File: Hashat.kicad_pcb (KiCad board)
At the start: 4 copper layers, 65 x 56.5 mm, 109 parts, among them IC1 BM1397_mode1, J1 Raspberry_Pi_2_3, J2 Conn_01x04, J3 Conn_01x05, Q1 CSD17311Q5, Q2 CSD17311Q5, U10 DS4432U+, U2 LN1134A182MR-G, U3 SN74LVC1T45DBVR, U4 SGM2036-ADJYN5G/TR, U5 SN74LVC1T45DBVR, U7 EMC2101-R, U8 SN74LVC1T45DBVR, U9 TPS40305, X1 OT322525MJBA4SL

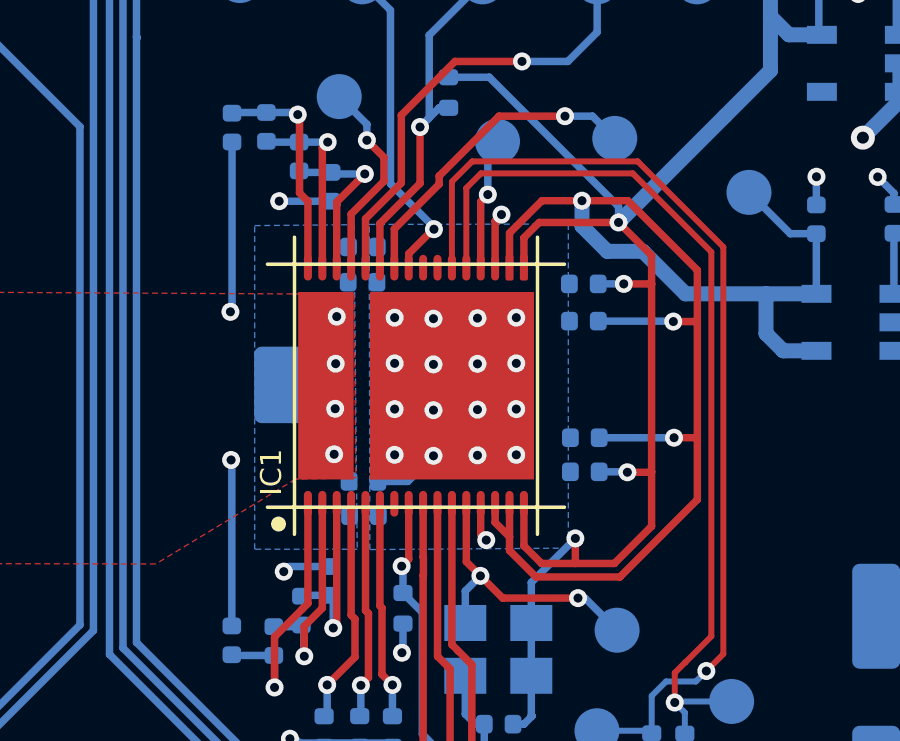
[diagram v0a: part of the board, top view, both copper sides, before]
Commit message: trace massaging
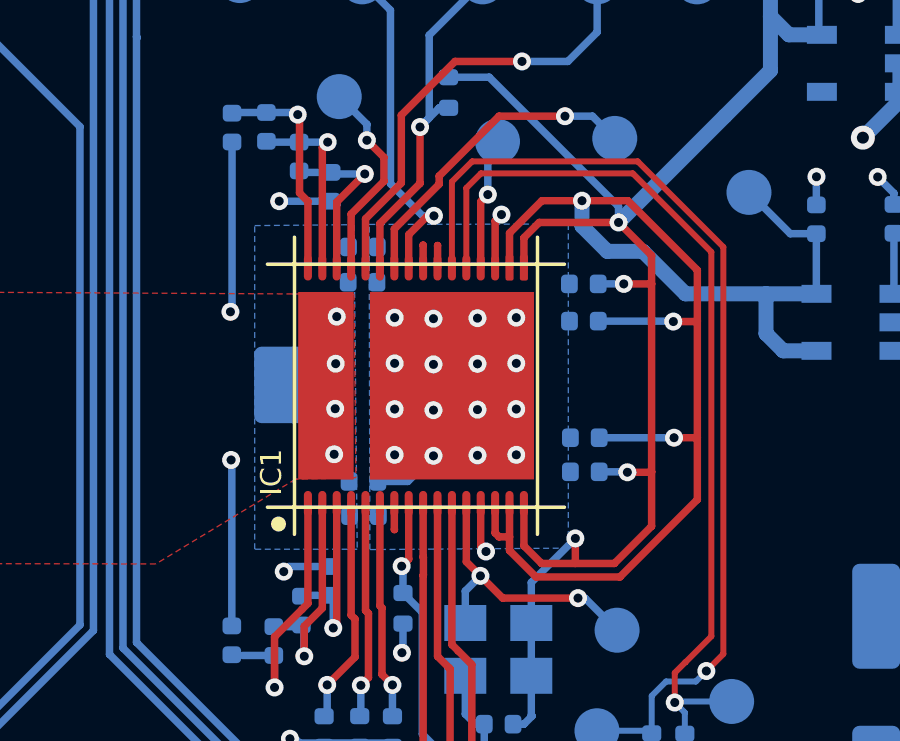
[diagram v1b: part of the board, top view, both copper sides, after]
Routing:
- net unconnected-(IC1-TEST-Pad7): track 0.00 -> 0.87 mm
- net unconnected-(IC1-TF-Pad24): track 0.00 -> 0.75 mm
- net unconnected-(IC1-RF-Pad23): track 0.00 -> 0.74 mm
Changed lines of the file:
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@@
   (segment (start 93.398 65.976) (end 92.085 65.976) (width 0.5) (layer "F.Cu") (net 1))
   (segment (start 119.9764 81.742026) (end 119.9764 83.2994) (width 0.25) (layer "F.Cu") (net 1))
+  (segment (start 119.672 92.76) (end 119.4964 92.5844) (width 0.25) (layer "F.Cu") (net 1))
   (segment (start 92.085 65.976) (end 91.554 65.445) (width 0.5) (layer "F.Cu") (net 1))
   (segment (start 120.188381 81.530045) (end 119.9764 81.742026) (width 0.25) (layer "F.Cu") (net 1))
-  (segment (start 119.4964 91.1686) (end 119.4964 92.1944) (width 0.25) (layer "F.Cu") (net 1))
-  (segment (start 119.4964 92.1944) (end 119.681 92.379) (width 0.25) (layer "F.Cu") (net 1))
+  (segment (start 119.4964 92.5844) (end 119.4964 91.1686) (width 0.25) (layer "F.Cu") (net 1))
   (via (at 108.847 104.527) (size 0.6) (drill 0.3) (layers "F.Cu" "B.Cu") (net 1))
   (via (at 90.763745 81.944278) (size 0.6) (drill 0.3) (layers "F.Cu" "B.Cu") (net 1))
@@
   (via (at 89.63 82.723) (size 0.6) (drill 0.3) (layers "F.Cu" "B.Cu") (net 1))
   (via (at 91.249 100.085) (size 0.6) (drill 0.3) (layers "F.Cu" "B.Cu") (net 1))
-  (via (at 119.681 92.379) (size 0.6) (drill 0.3) (layers "F.Cu" "B.Cu") (net 1))
+  (via (at 119.672 92.76) (size 0.6) (drill 0.3) (layers "F.Cu" "B.Cu") (net 1))
   (via (at 120.682 84.964) (size 0.6) (drill 0.3) (layers "F.Cu" "B.Cu") (net 1))
   (via (at 117.921 88.046666) (size 0.6) (drill 0.3) (layers "F.Cu" "B.Cu") (net 1))
@@
   (segment (start 121.337604 93.608) (end 124.138396 93.608) (width 0.25) (layer "F.Cu") (net 36))
   (segment (start 124.4025 81.0665) (end 122.872 81.0665) (width 0.25) (layer "F.Cu") (net 36))
-  (segment (start 119.9764 91.1686) (end 119.9764 91.791) (width 0.25) (layer "F.Cu") (net 36))
   (segment (start 126.717 88.967) (end 126.717 85.08) (width 0.25) (layer "F.Cu") (net 36))
   (segment (start 126.717 85.08) (end 126.717 83.381) (width 0.25) (layer "F.Cu") (net 36))
+  (segment (start 119.9764 91.1686) (end 119.9764 92.1404) (width 0.25) (layer "F.Cu") (net 36))
+  (segment (start 120.107 92.271) (end 120.4564 92.271) (width 0.25) (layer "F.Cu") (net 36))
   (segment (start 120.4564 82.145204) (end 121.535104 81.0665) (width 0.25) (layer "F.Cu") (net 36))
   (segment (start 125.94 88.967) (end 126.717 88.967) (width 0.25) (layer "F.Cu") (net 36))
+  (segment (start 119.9764 92.1404) (end 120.107 92.271) (width 0.25) (layer "F.Cu") (net 36))
   (segment (start 121.535104 81.0665) (end 122.872 81.0665) (width 0.25) (layer "F.Cu") (net 36))
   (segment (start 120.4564 92.726796) (end 121.337604 93.608) (width 0.25) (layer "F.Cu") (net 36))
@@
   (segment (start 124.138396 93.608) (end 126.717 91.029396) (width 0.25) (layer "F.Cu") (net 36))
   (segment (start 120.4564 83.2994) (end 120.4564 82.145204) (width 0.25) (layer "F.Cu") (net 36))
-  (segment (start 119.9764 91.791) (end 120.4564 92.271) (width 0.25) (layer "F.Cu") (net 36))
   (segment (start 125.9165 85.095) (end 126.702 85.095) (width 0.25) (layer "F.Cu") (net 36))
   (segment (start 126.717 83.381) (end 124.4025 81.0665) (width 0.25) (layer "F.Cu") (net 36))
@@
   (via (at 116.554 97.207) (size 0.6) (drill 0.3) (layers "F.Cu" "B.Cu") (net 43))
   (segment (start 116.554 97.207) (end 116.554 98.251) (width 0.25) (layer "B.Cu") (net 43))
+  (segment (start 116.6164 91.1686) (end 116.6164 92.0264) (width 0.25) (layer "F.Cu") (net 44))
+  (segment (start 116.6164 92.0264) (end 116.622 92.032) (width 0.25) (layer "F.Cu") (net 44))
   (segment (start 117.0964 93.0135) (end 117.0964 91.1686) (width 0.25) (layer "F.Cu") (net 45))
   (segment (start 116.8609 93.249) (end 117.0964 93.0135) (width 0.25) (layer "F.Cu") (net 45))
@@
   (segment (start 125.196 97.570794) (end 125.196 98.822) (width 0.2) (layer "B.Cu") (net 48))
   (segment (start 125.108 98.734) (end 125.196 98.822) (width 0.2) (layer "B.Cu") (net 48))
-  (segment (start 117.9369 82.016) (end 117.914262 82.016) (width 0.25) (layer "F.Cu") (net 51))
-  (segment (start 117.914262 82.016) (end 117.0964 82.833862) (width 0.25) (layer "F.Cu") (net 51))
-  (segment (start 117.0964 82.833862) (end 117.0964 83.2994) (width 0.25) (layer "F.Cu") (net 51))
-  (via (at 117.9369 82.016) (size 0.6) (drill 0.3) (layers "F.Cu" "B.Cu") (net 51))
+  (segment (start 118.058 83.2978) (end 118.058 82.561) (width 0.25) (layer "F.Cu") (net 49))
+  (segment (start 118.058 82.561) (end 118.06 82.559) (width 0.25) (layer "F.Cu") (net 49))
+  (segment (start 118.0564 83.2994) (end 118.058 83.2978) (width 0.25) (layer "F.Cu") (net 49))
+  (segment (start 117.5764 82.5484) (end 117.574 82.546) (width 0.25) (layer "F.Cu") (net 50))
+  (segment (start 117.5764 83.2994) (end 117.5764 82.5484) (width 0.25) (layer "F.Cu") (net 50))
+  (segment (start 117.0964 82.1976) (end 117.0964 83.2994) (width 0.25) (layer "F.Cu") (net 51))
+  (segment (start 117.722723 81.571277) (end 117.0964 82.1976) (width 0.25) (layer "F.Cu") (net 51))
+  (segment (start 117.9369 81.571277) (end 117.722723 81.571277) (width 0.25) (layer "F.Cu") (net 51))
+  (via (at 117.9369 81.571277) (size 0.6) (drill 0.3) (layers "F.Cu" "B.Cu") (net 51))
+  (segment (start 116.488 80.501) (end 116.488 74.716) (width 0.25) (layer "B.Cu") (net 51))
   (segment (start 116.488 74.716) (end 115.543 73.771) (width 0.25) (layer "B.Cu") (net 51))
-  (segment (start 117.9369 82.016) (end 117.9369 81.9499) (width 0.25) (layer "B.Cu") (net 51))
-  (segment (start 116.488 80.501) (end 116.488 74.716) (width 0.25) (layer "B.Cu") (net 51))
-  (segment (start 117.9369 81.9499) (end 116.488 80.501) (width 0.25) (layer "B.Cu") (net 51))
+  (segment (start 117.9369 81.571277) (end 117.558277 81.571277) (width 0.25) (layer "B.Cu") (net 51))
+  (segment (start 117.558277 81.571277) (end 116.488 80.501) (width 0.25) (layer "B.Cu") (net 51))
   (segment (start 118.1114 80.5136) (end 118.1114 80.2446) (width 0.25) (layer "F.Cu") (net 52))
   (segment (start 118.1114 80.2446) (end 120.107 78.249) (width 0.25) (layer "F.Cu") (net 52))
